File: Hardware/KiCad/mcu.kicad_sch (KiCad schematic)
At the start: 10 parts, among them U3 STM32F427ZGTx, Y1 8 MHz, Y2 32 kHz

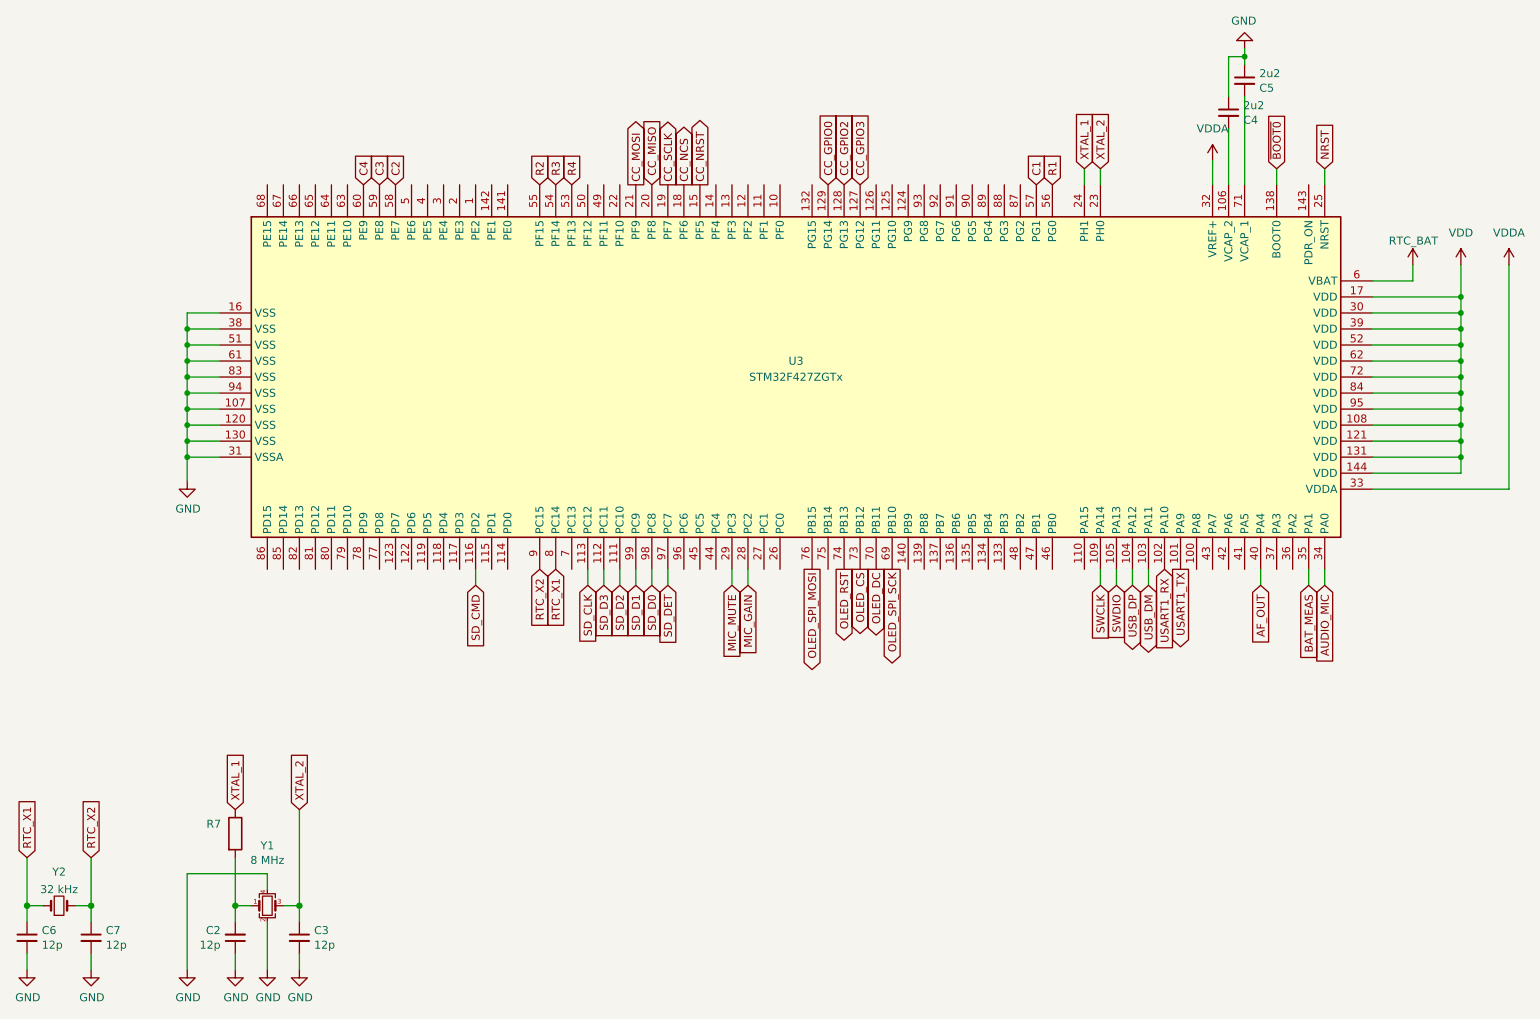
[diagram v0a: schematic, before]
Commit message: R7 update
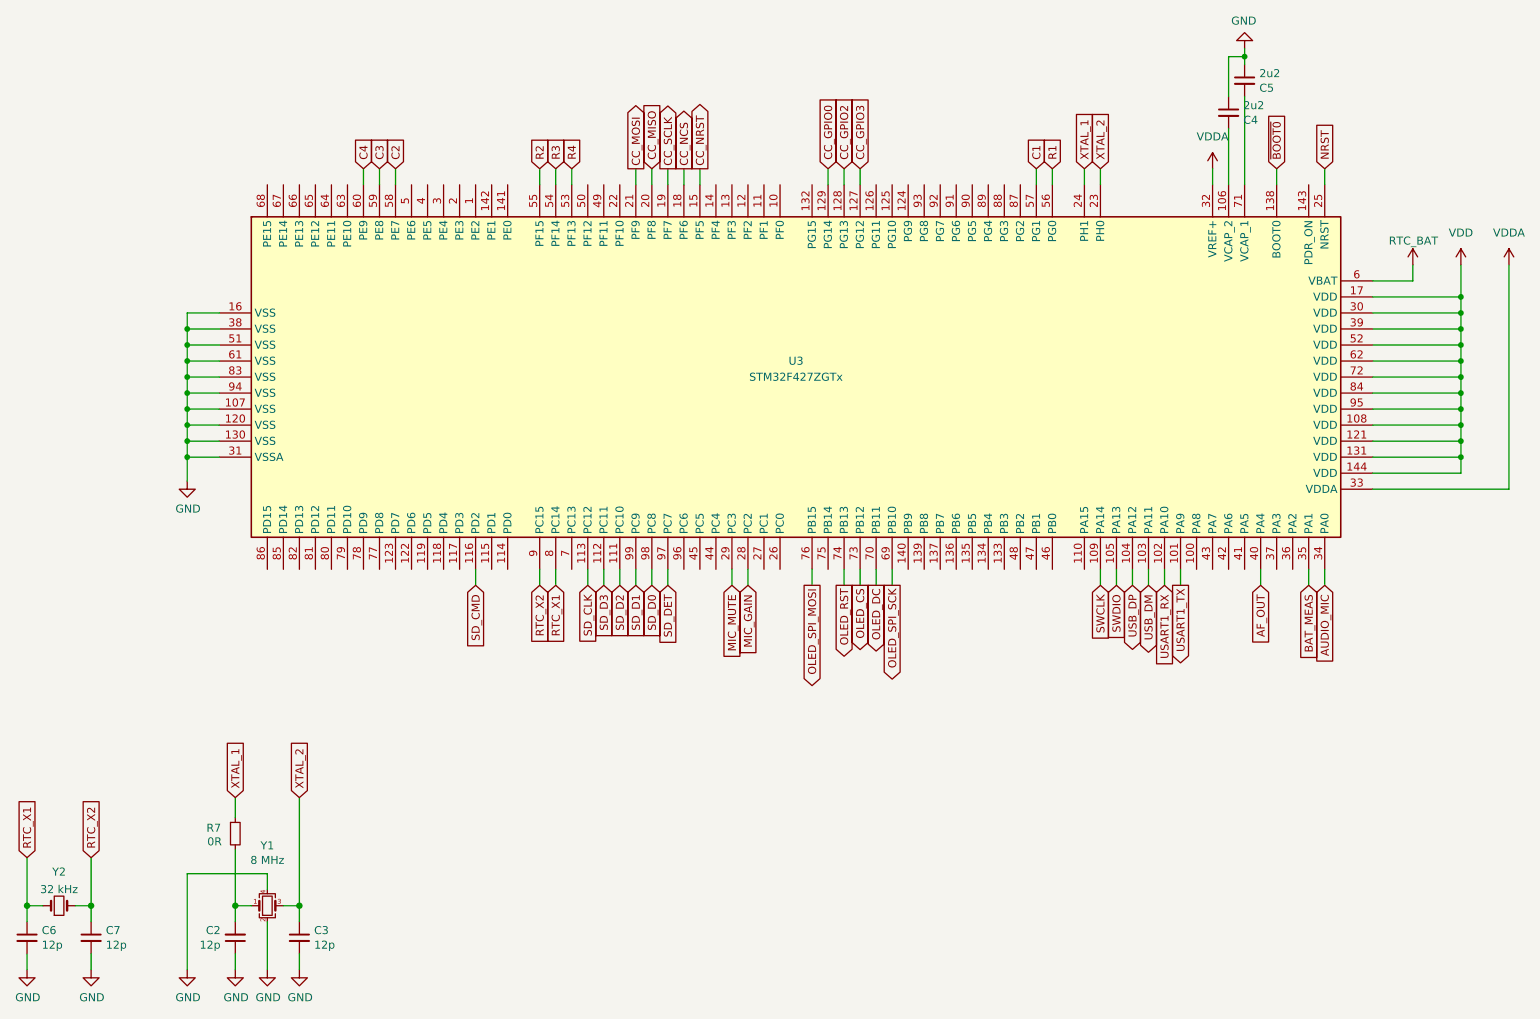
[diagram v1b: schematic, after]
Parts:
- R7: value (none) -> 0R; footprint (none) -> Resistor_SMD:R_0402_1005Metric; symbol Device:R -> Device:R_Small
